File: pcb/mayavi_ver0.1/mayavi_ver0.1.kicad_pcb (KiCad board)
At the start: 2 copper layers, 31.5 x 32 mm, 25 parts, among them J1 3.7V LiPo, J2 Charging Conn, J3 OLED Connector, J4 CONN_01X04, SW1 SW_Push, SW2 SW_Push, SW3 SW_Push, U1 MCP1702, U2 LIS2DH12, U3 MDBT42V

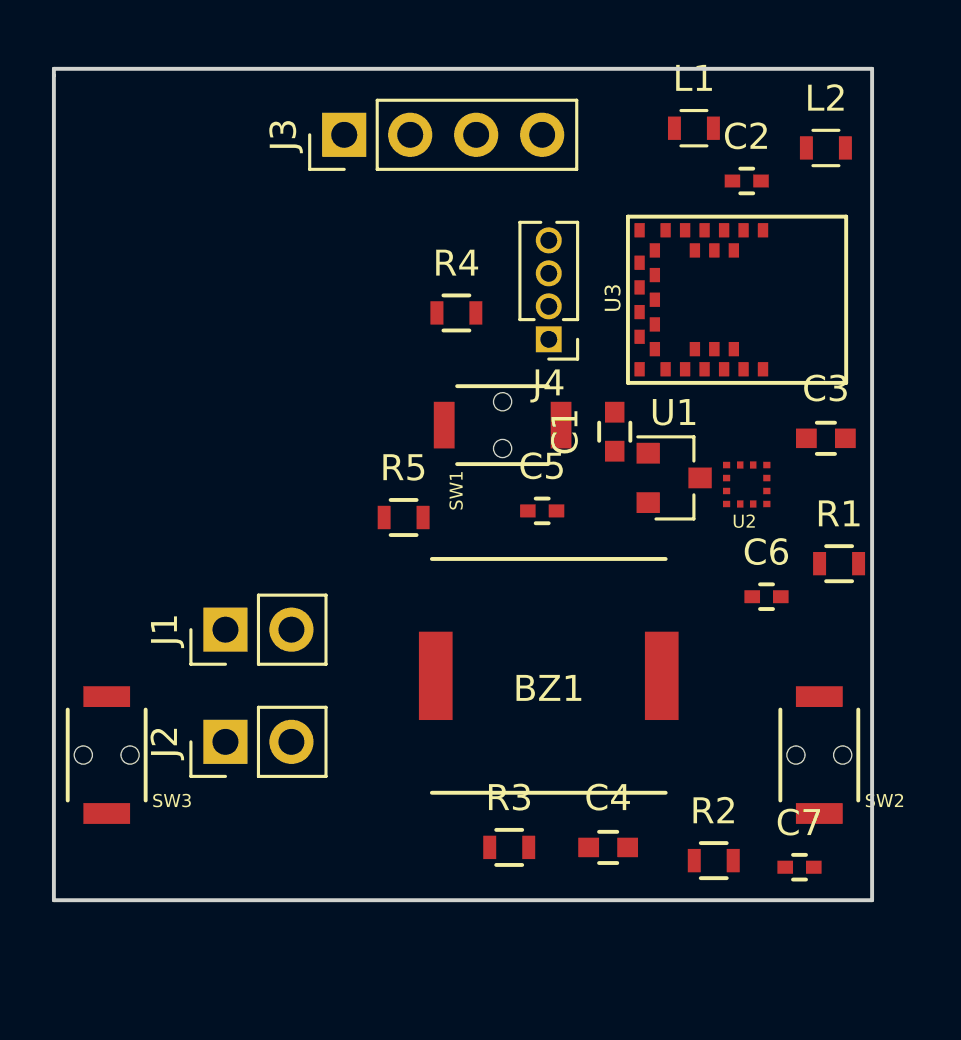
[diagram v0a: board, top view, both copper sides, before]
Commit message: updated pcb
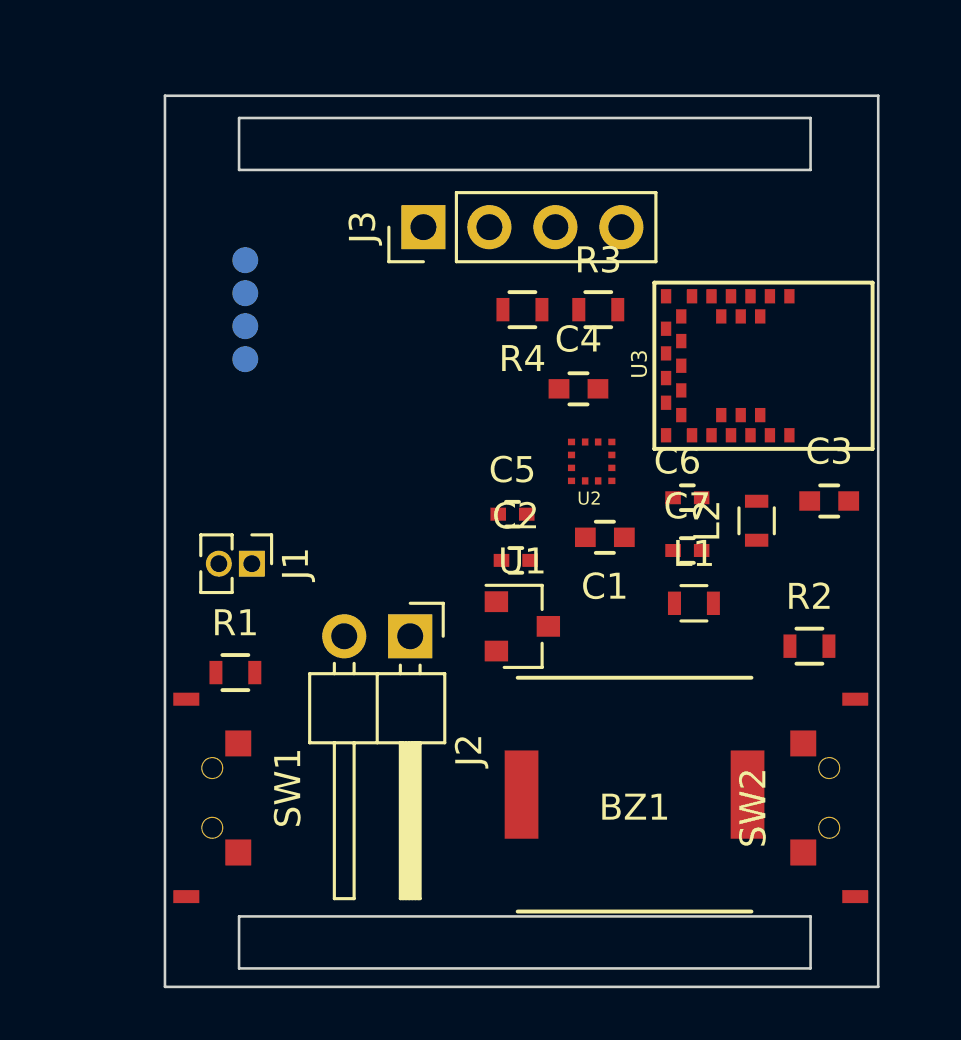
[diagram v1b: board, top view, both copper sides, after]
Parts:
- removed R5: 10K, Resistors_SMD:R_0603
- removed SW3: SW_Push, mayavi:peter-switch
- J1: footprint Pin_Headers:Pin_Header_Straight_1x02_Pitch2.54mm -> Pin_Headers:Pin_Header_Straight_1x02_Pitch1.27mm
- J2: footprint Pin_Headers:Pin_Header_Straight_1x02_Pitch2.54mm -> Pin_Headers:Pin_Header_Angled_1x02_Pitch2.54mm
- J4: value CONN_01X04 -> SWD header; footprint Pin_Headers:Pin_Header_Straight_1x04_Pitch1.27mm -> mayavi:SWD_1.27; moved to B.Cu
- SW1, SW2: footprint mayavi:peter-switch -> mayavi:SW5052
- moved R1 23.6 mm to (114.4, 86.0)
- moved R3 21.0 mm to (128.4, 72.0)
- moved L1 18.3 mm to (132.1, 83.3)
- moved SW1 18.2 mm to (113.5, 90.8), turned to 90 degrees
- moved C4 17.7 mm to (127.6, 75.1)
- moved C2 17.1 mm to (125.2, 81.7)
- moved L2 14.6 mm to (134.5, 80.1), turned to 90 degrees
- moved C7 12.9 mm to (131.8, 81.3)
- moved J4 12.1 mm to (114.8, 70.1)
- moved R2 9.04 mm to (136.5, 85.0)
- moved J2 8.19 mm to (121.2, 84.6), turned to 270 degrees
- moved U1 8.17 mm to (125.5, 84.2)
- moved U2 6.03 mm to (128.1, 77.9)
- moved BZ1 5.64 mm to (129.8, 90.7)
- moved C6 4.88 mm to (131.8, 79.2)
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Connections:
- R1 pad 2: RESET -> BTN1
- R2 pad 2: BTN1 -> BTN2
- R3 pad 2: BTN2 -> SDA
- R4 pad 2: SDA -> SCL
- U3 pad 3: RESET -> (no net)
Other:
- board size 31.5 x 32 mm -> 27.5 x 34.3 mm
- board text added: "Mayavi"
